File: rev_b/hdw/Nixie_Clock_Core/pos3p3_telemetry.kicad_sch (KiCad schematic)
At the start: 7 parts

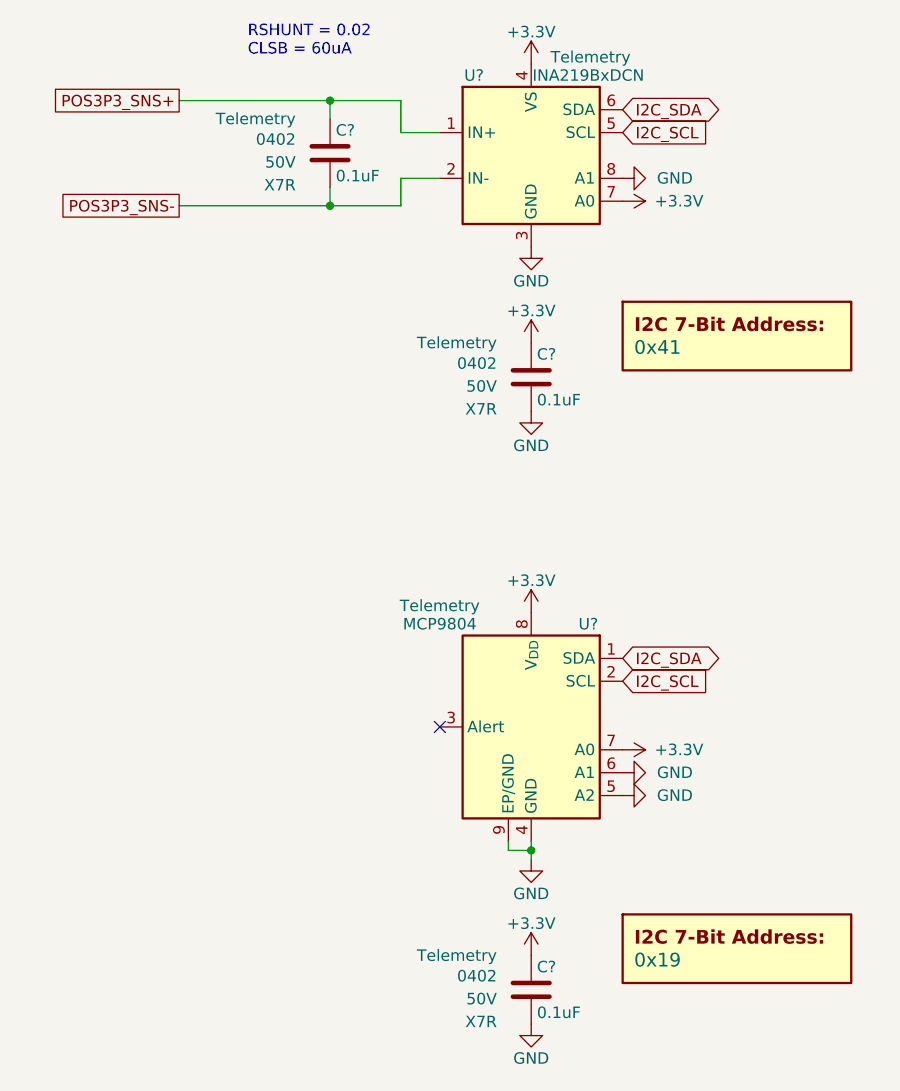
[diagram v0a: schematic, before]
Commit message: more rev b sch progress
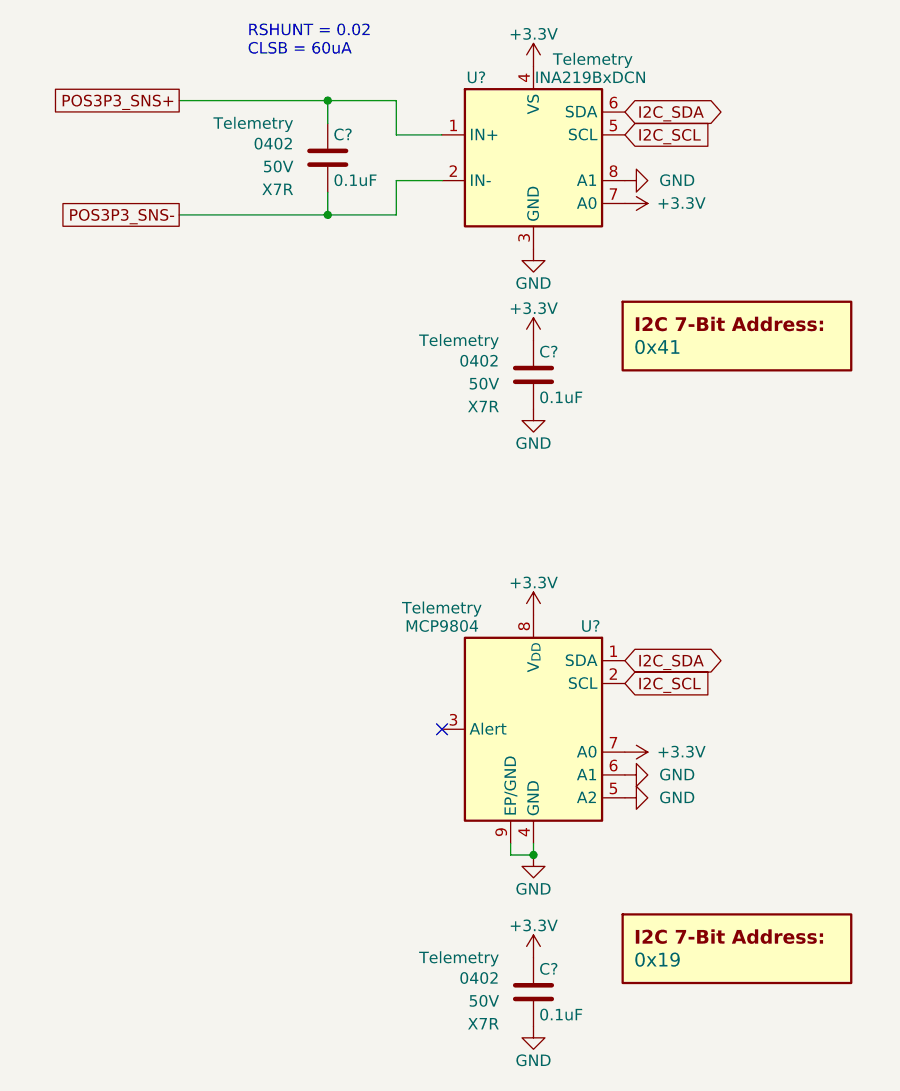
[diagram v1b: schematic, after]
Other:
- moved on the sheet: C?
